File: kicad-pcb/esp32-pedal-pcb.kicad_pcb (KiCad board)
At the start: 4 copper layers, 216 x 25 mm, 40 parts, among them J1 USB_C_Receptacle_USB2.0_14P, Q1 Q_PMOS_GSD, U1 MCP73871, U2 TLV75733PDBV, U3 ESP32-S3-WROOM-1, U4 TPD2EUSB30, U5 TPD2E2U06DCK

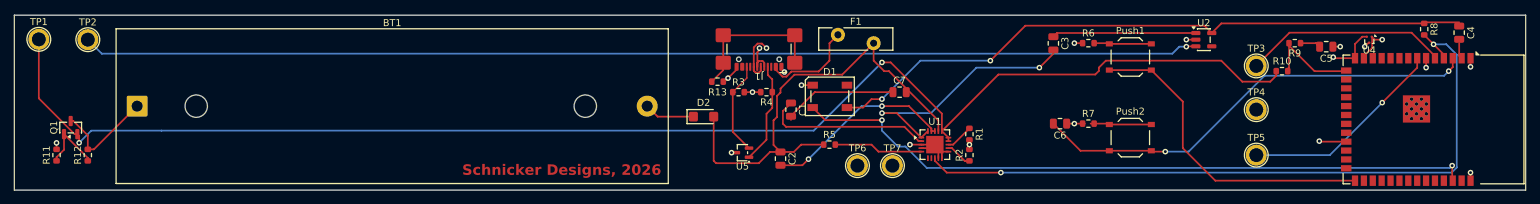
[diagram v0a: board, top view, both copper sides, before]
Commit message: Update PCB design, documentation, and images
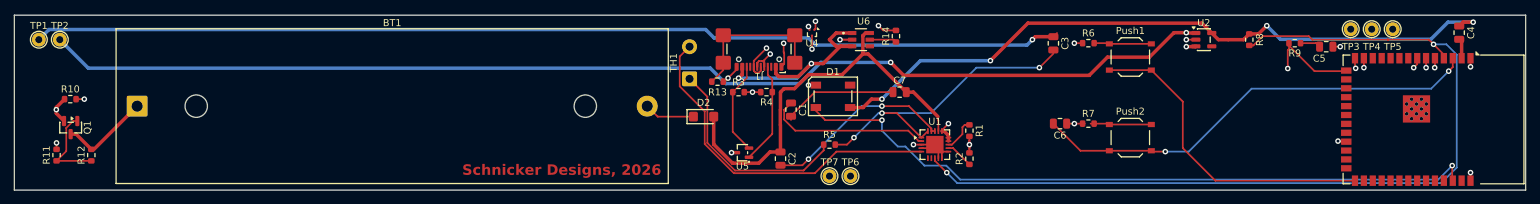
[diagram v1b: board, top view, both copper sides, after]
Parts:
- removed F1: Polyfuse_Small, Fuse:Fuse_Bourns_MF-RG500
- added R14: 100kΩ, Resistor_SMD:R_0603_1608Metric, F.Cu at (159.5, 90.5)
- added TH1: Thermistor_NTC_US, Connector_Wire:SolderWire-0.5sqmm_1x02_P4.6mm_D0.9mm_OD2.1mm, F.Cu at (130.0, 96.6)
- added U6: TPS2553DBVR, TPS2553DBVR:SOT95P280X145-6N, F.Cu at (154.5, 91.0)
- TP1: value R+ -> TestPoint_Small; footprint TestPoint:TestPoint_Plated_Hole_D2.0mm -> TestPoint:TestPoint_THTPad_D2.0mm_Drill1.0mm
- TP2: value R- -> TestPoint_Small; footprint TestPoint:TestPoint_Plated_Hole_D2.0mm -> TestPoint:TestPoint_THTPad_D2.0mm_Drill1.0mm
- TP3, TP6: value SW1 -> TestPoint_Small; footprint TestPoint:TestPoint_Plated_Hole_D2.0mm -> TestPoint:TestPoint_THTPad_D2.0mm_Drill1.0mm
- TP4, TP7: value SW GND -> TestPoint_Small; footprint TestPoint:TestPoint_Plated_Hole_D2.0mm -> TestPoint:TestPoint_THTPad_D2.0mm_Drill1.0mm
- TP5: value SW2 -> TestPoint_Small; footprint TestPoint:TestPoint_Plated_Hole_D2.0mm -> TestPoint:TestPoint_THTPad_D2.0mm_Drill1.0mm
- moved R10 173.2 mm to (41.5, 99.5)
- moved U4 79.7 mm to (147.5, 90.0)
- moved TP5 26.5 mm to (230.5, 89.5)
- moved R8 25.0 mm to (210.0, 91.0)
- moved TP4 20.1 mm to (227.5, 89.5)
- moved TP3 14.5 mm to (224.5, 89.5)
- moved TP7 9.12 mm to (150.0, 110.5)
- moved TP2 4.00 mm to (40.0, 91.0)
- moved TP6 1.80 mm to (153.0, 110.5)
- moved R1 0.50 mm to (170.0, 104.0)
- moved R12 0.50 mm to (44.5, 107.5)
- moved R2 0.50 mm to (170.0, 108.0)
- moved D1 0.45 mm to (150.5, 99.1)
- turned Q1 to -90 degrees
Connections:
- C3 pad 1: Net-(U2-IN) -> Net-(C3-Pad1)
- Q1 pad 2: /BAT PROTECTED -> /VBAT
- R10 pad 1: /BAT PROTECTED -> /VBAT
- R5 pad 1: /VBUS PROTECTED -> Net-(R5-Pad1)
- R5 pad 2: Net-(U1-THERM) -> Net-(C3-Pad2)
- TP1 pad 1: /BAT PROTECTED -> Net-(C3-Pad1)
- TP2 pad 1: /BAT PROTECTED -> /BAT SWITCHED
- U1 pad 14: /BAT PROTECTED -> /VBAT
- U1 pad 15: /BAT PROTECTED -> /VBAT
- U1 pad 16: /BAT PROTECTED -> /VBAT
- U2 pad 1: Net-(U2-IN) -> /BAT SWITCHED
- U2 pad 3: /BAT PROTECTED -> /BAT SWITCHED
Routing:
- net /BAT PROTECTED: track 366.9 -> 0.00 mm, vias 3 -> 0
- net Net-(U3-GPIO3/TOUCH3/ADC1_CH2): track 13.9 -> 189.8 mm, vias 0 -> 2
- net /BAT SWITCHED: track 0.00 -> 173.8 mm, vias 0 -> 3
- net Net-(C3-Pad1): track 0.00 -> 147.8 mm, vias 0 -> 1
- net /VBAT: track 0.00 -> 136.7 mm, vias 0 -> 2
- net Net-(U1-THERM): track 12.5 -> 49.9 mm
- net Net-(R5-Pad1): track 0.00 -> 30.0 mm
- net Net-(U1-STAT1/~{LBO}): track 100.9 -> 127.6 mm
- net Net-(U3-GPIO7/TOUCH7/ADC1_CH6): track 29.5 -> 8.30 mm
- net /VBUS: track 13.6 -> 34.3 mm, vias 0 -> 2
- net Net-(U2-IN): track 20.6 -> 0.00 mm
- net Net-(U3-GPIO5/TOUCH5/ADC1_CH4): track 29.2 -> 16.5 mm, vias 0 -> 1
- net Net-(C3-Pad2): track 36.4 -> 45.0 mm, vias 2 -> 3
- net /VBUS PROTECTED: track 65.9 -> 58.2 mm
- net /GND: track 46.5 -> 53.5 mm, vias 16 -> 18
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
